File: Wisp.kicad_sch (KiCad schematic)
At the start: 36 parts, among them J1 USB4105-GF-A, J2 SM04B-GHS-TB, J6 Conn_01x04_Pin, J9 Conn_02x04_Counter_Clockwise, SW2 PTS810 SJM 250 SMTR LFS, SW3 PTS810 SJM 250 SMTR LFS, T1 UTX, U1 ESP32-S3-MINI-1, U2 USBLC6-2SC6, U3 AP2112K-3.3TRG1, U4 TPS7A2033PDBVR, U5 DWM3000TR13

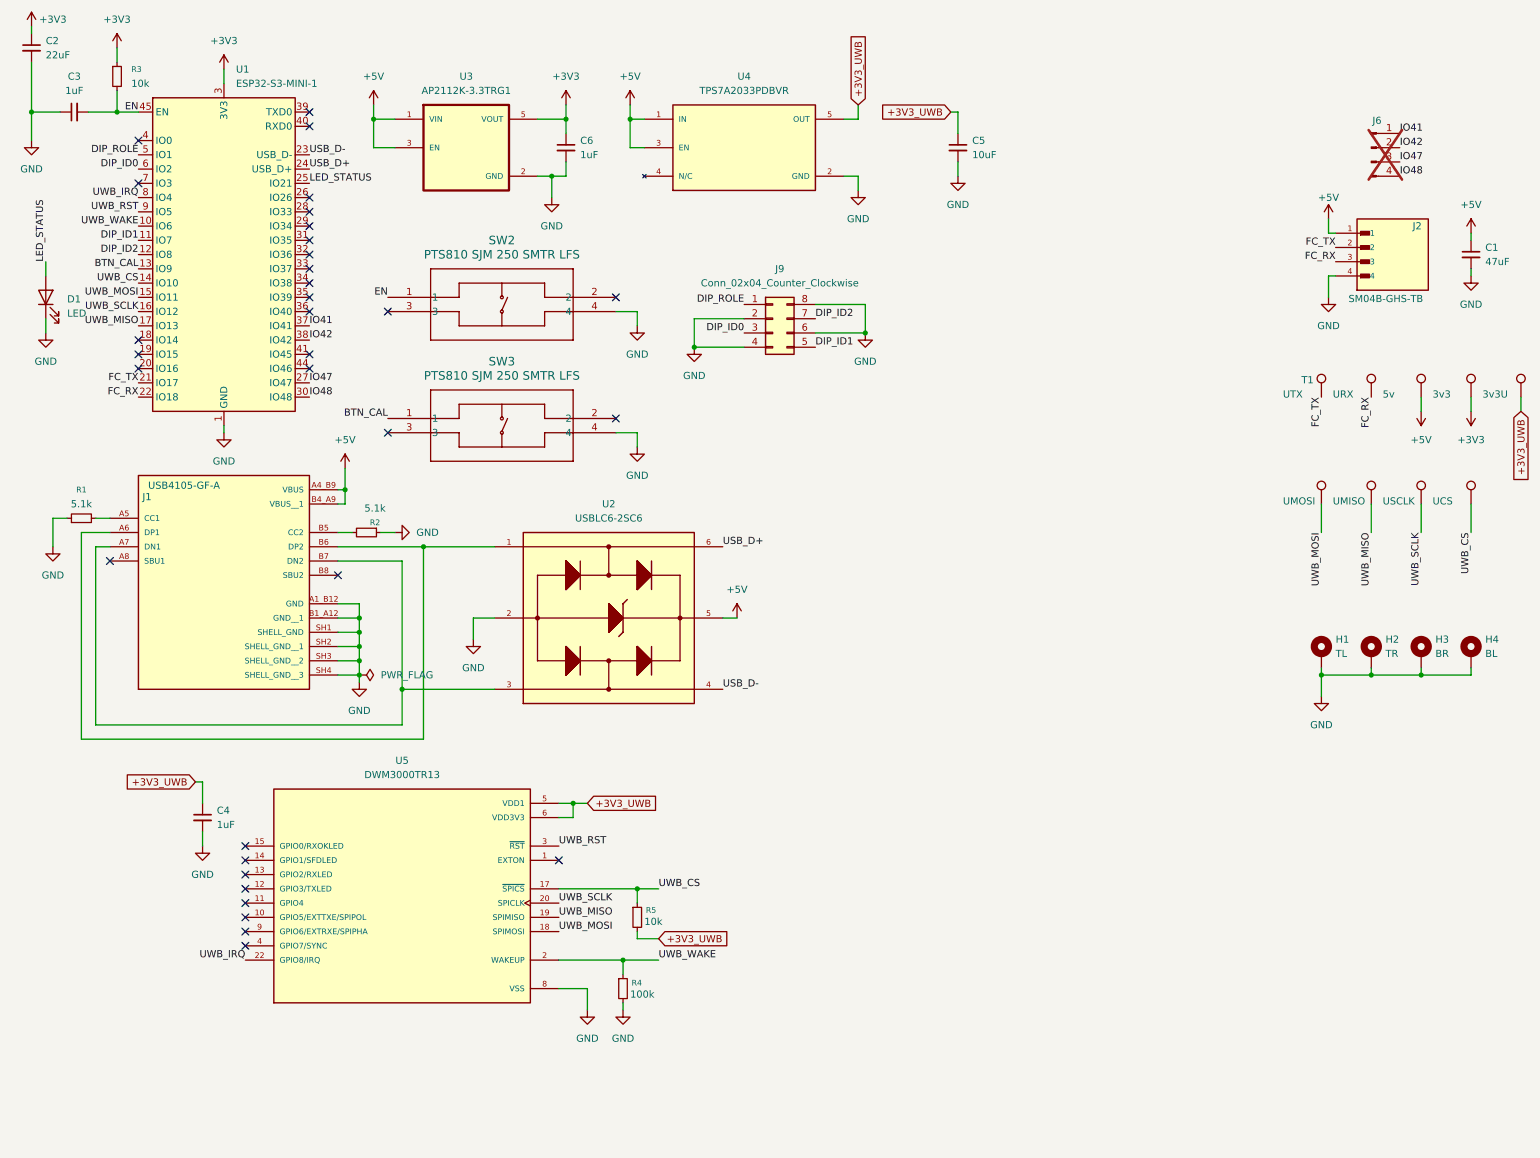
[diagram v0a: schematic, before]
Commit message: Organized the schematic into sections
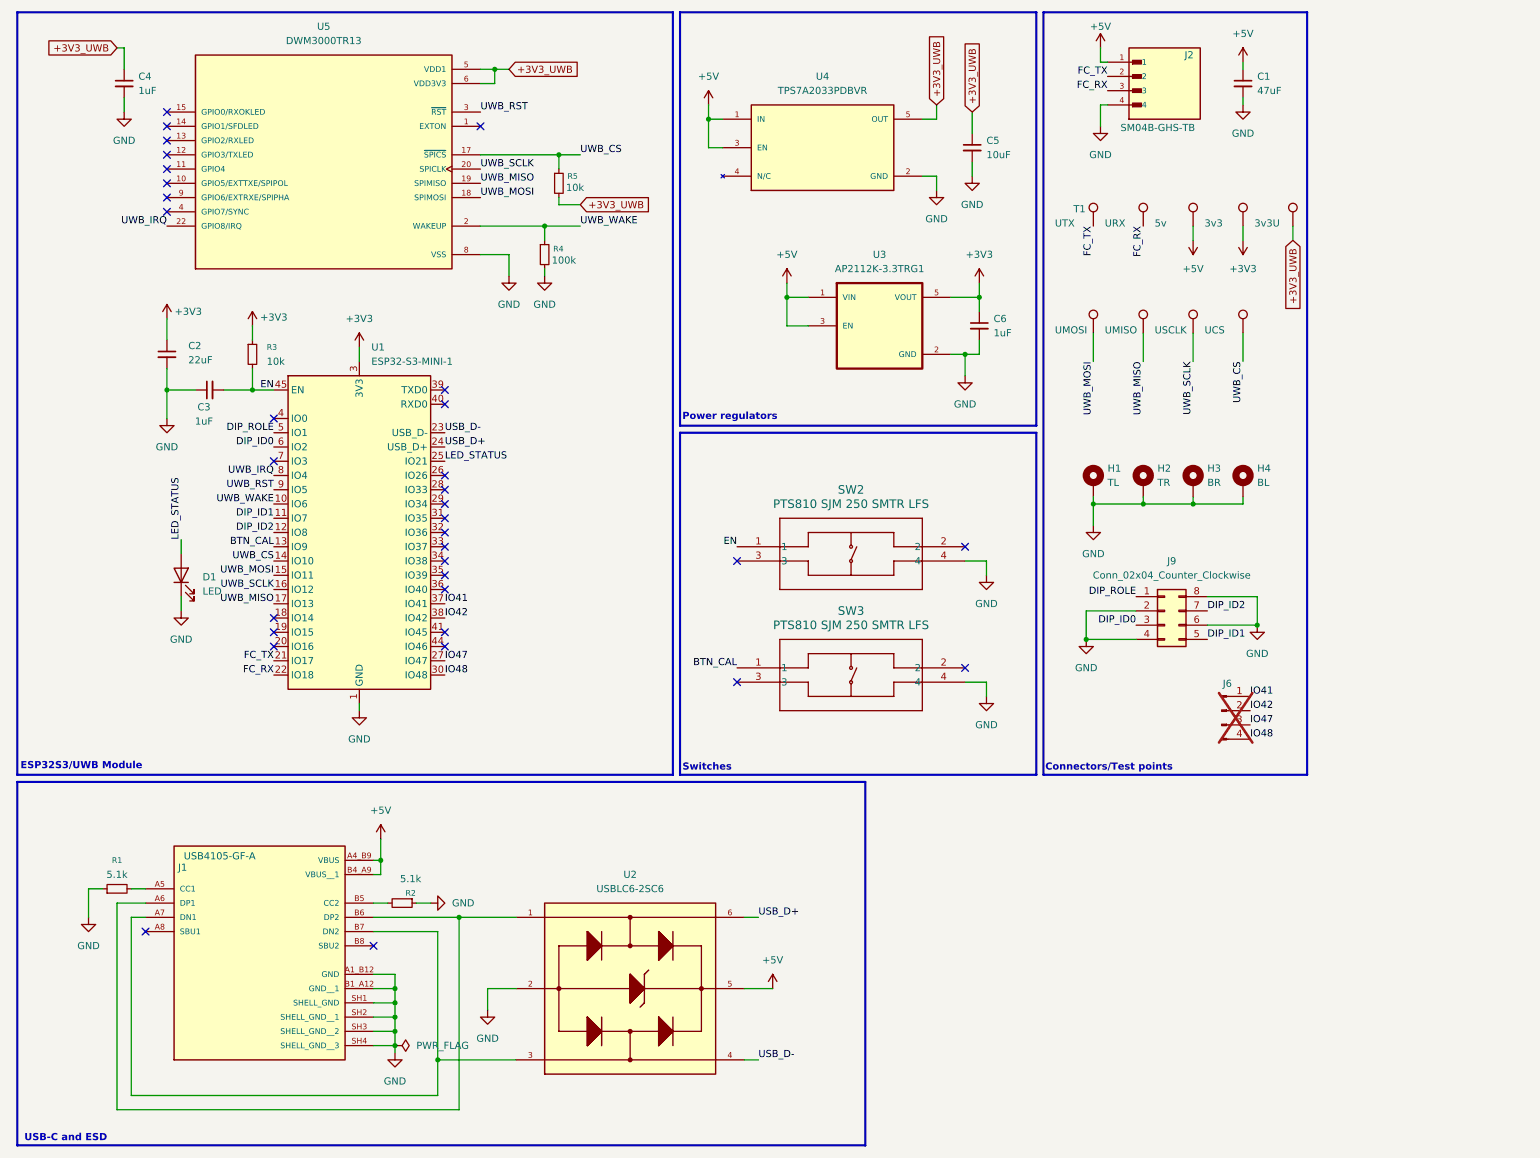
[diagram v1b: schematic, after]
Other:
- note added: "Connectors/Test points"
- note added: "ESP32S3/UWB Module"
- note added: "Power regulators"
- note added: "Switches"
- note added: "USB-C and ESD"
- moved on the sheet: C1, C2, C3, C4, C5, C6, D1, H1, H2, H3, H4, J1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
